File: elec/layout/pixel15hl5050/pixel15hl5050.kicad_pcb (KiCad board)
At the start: 2 copper layers, 5 parts

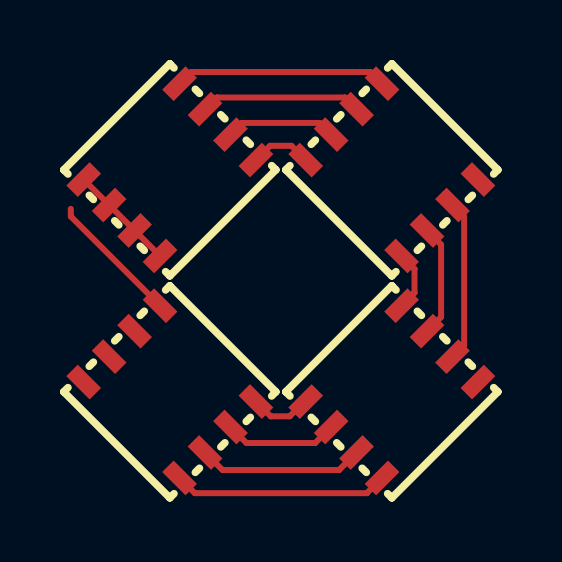
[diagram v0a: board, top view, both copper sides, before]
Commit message: tight layout
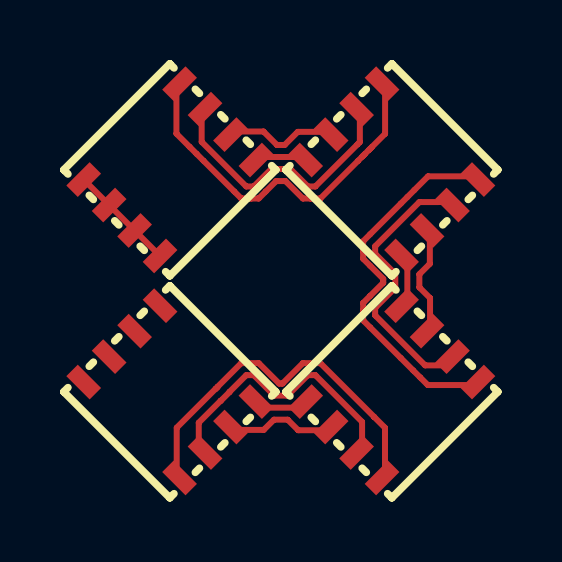
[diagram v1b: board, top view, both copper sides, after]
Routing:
- net rgbs[2]-anodes-anode-1: track 0.00 -> 12.3 mm
- net rgbs[3]-anodes-anode-1: track 7.17 -> 12.8 mm
- net rgbs[1]-anodes-anode-1: track 7.07 -> 12.6 mm
- net rgbs[3]-cathodes-cathode-3: track 4.46 -> 0.00 mm
- net rgbs[2]-anodes-anode-0: track 5.37 -> 9.48 mm
- net rgbs[3]-anodes-anode-0: track 5.54 -> 9.49 mm
- net rgbs[1]-anodes-anode-0: track 5.37 -> 9.26 mm
